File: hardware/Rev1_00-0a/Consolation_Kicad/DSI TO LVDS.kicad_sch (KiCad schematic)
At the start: 27 parts, among them Q10 SSM3K56FS,LF, Q11 SSM3K56FS,LF, U15 SN65DSI84ZXHR, U16 SN74LVC1G125DBVR

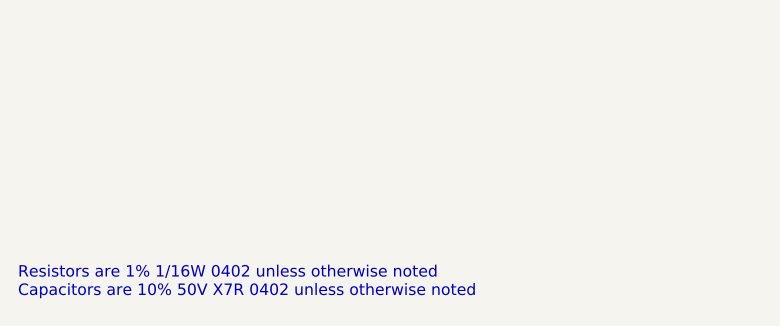
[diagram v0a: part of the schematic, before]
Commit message: Update schematics, block diagram and pin mux (good progress G)
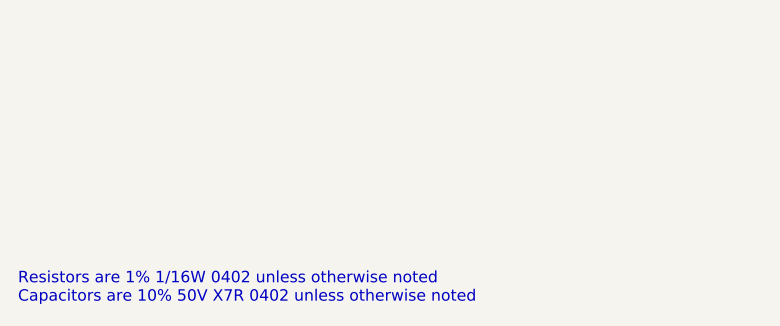
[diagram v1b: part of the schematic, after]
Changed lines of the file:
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@@
 	(text "Resistors are 1% 1/16W 0402 unless otherwise noted\nCapacitors are 10% 50V X7R 0402 unless otherwise noted"
 		(exclude_from_sim no)
-		(at 12.7 170.307 0)
+		(at 12.7 170.942 0)
 		(effects
 			(font
